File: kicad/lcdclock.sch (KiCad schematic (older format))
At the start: 24 parts, among them J1 Conn_JLink_SWD, SW1 SW_Push, U1 STM32L073xx_48, U2 ELV_DCF-2, U3 TPS70630, U4 LCD, Y1 32.768kHz 12.5pF

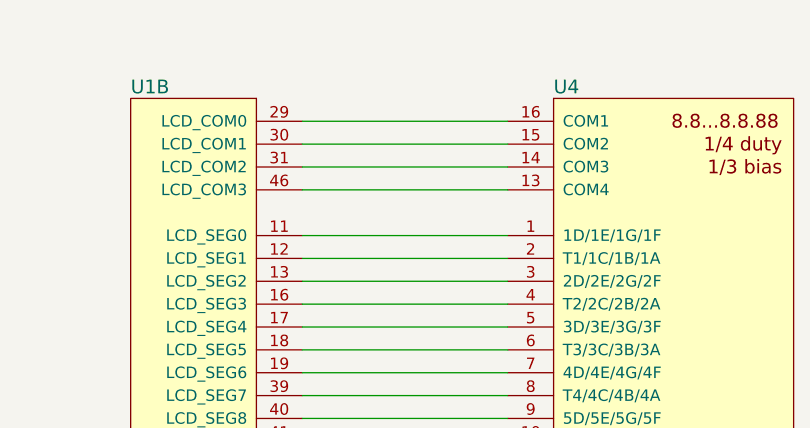
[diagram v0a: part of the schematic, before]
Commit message: Layout PCB
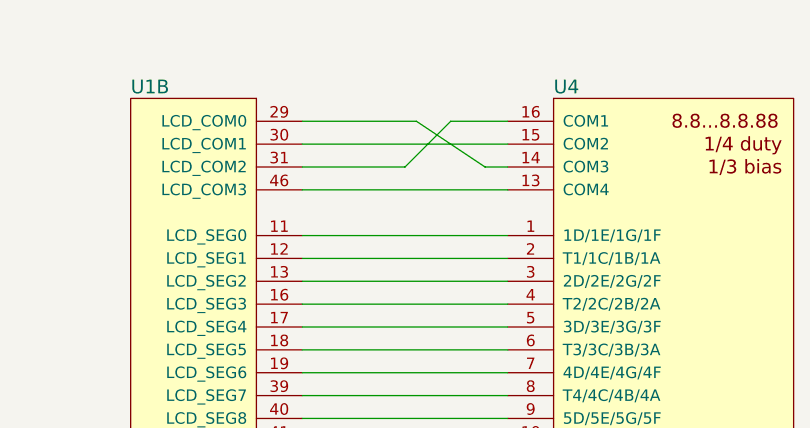
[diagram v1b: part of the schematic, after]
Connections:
- wire segments 103 -> 107
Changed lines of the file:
@@
 Connection ~ 5950 1550
-Wire Wire Line
-	8600 1300 9500 1300
-Wire Wire Line
-	8600 1400 9500 1400
-Wire Wire Line
-	8600 1500 9500 1500
-Wire Wire Line
-	8600 1600 9500 1600
 Wire Wire Line
 	8600 1800 9500 1800
@@
 	0    1    1    0
 $EndComp
+Wire Wire Line
+	8600 1600 9500 1600
+Wire Wire Line
+	8600 1400 9500 1400
+Wire Wire Line
+	8600 1300 9100 1300
+Wire Wire Line
+	9400 1500 9500 1500
+Wire Wire Line
+	9100 1300 9400 1500
+Wire Wire Line
+	8600 1500 9050 1500
+Wire Wire Line
+	9050 1500 9250 1300
+Wire Wire Line
+	9250 1300 9500 1300
 $EndSCHEMATC
